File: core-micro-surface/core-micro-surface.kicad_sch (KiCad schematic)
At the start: 140 parts, among them J1 SWD, J2 AudioPlug2, J3 USB_B, J4 Screw_Terminal_01x04, SW1 SW_Push, SW10 SW_Push, SW11 SW_Push, SW12 SW_Push, SW13 SW_Push, SW14 SW_Push, SW15 SW_Push, SW16 SW_Push, SW17 SW_Push, SW18 SW_Push, SW19 SW_Push, SW2 SW_Push, SW20 SW_Push, SW21 SW_Push, SW22 SW_Push, SW23 SW_Push, SW24 SW_Push, SW25 SW_Push, SW26 SW_Push, SW27 SW_Push, SW28 SW_Push, SW29 SW_Push, SW3 SW_Push, SW30 SW_Push, SW31 SW_Push, SW32 SW_Push, SW33 SW_Push, SW34 SW_Push, SW35 SW_Push, SW36 SW_Push, SW37 SW_Push, SW38 SW_Push, SW39 SW_Push, SW4 SW_Push, SW40 SW_Push, SW41 SW_Push, SW42 SW_Push, SW43 SW_Push, SW44 SW_Push, SW45 SW_Push, SW46 RotaryEncoder_Switch, SW47 RotaryEncoder_Switch, SW48 RotaryEncoder_Switch, SW5 SW_Push, SW6 SW_Push, SW7 SW_Push, SW8 SW_Push, SW9 SW_Push, U1 RP2040, U2 W25Q128JVS, U3 XC6206PxxxMR-Regulator_Linear, U4 USBLC6-2SC6, U5 ADS1115IDGS, Y1 12MHz

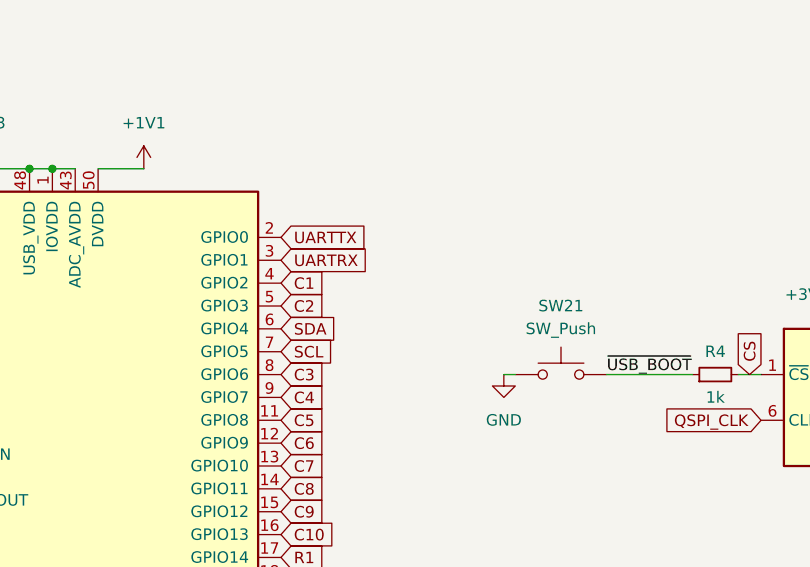
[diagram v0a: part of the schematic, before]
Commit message: Various things were completed
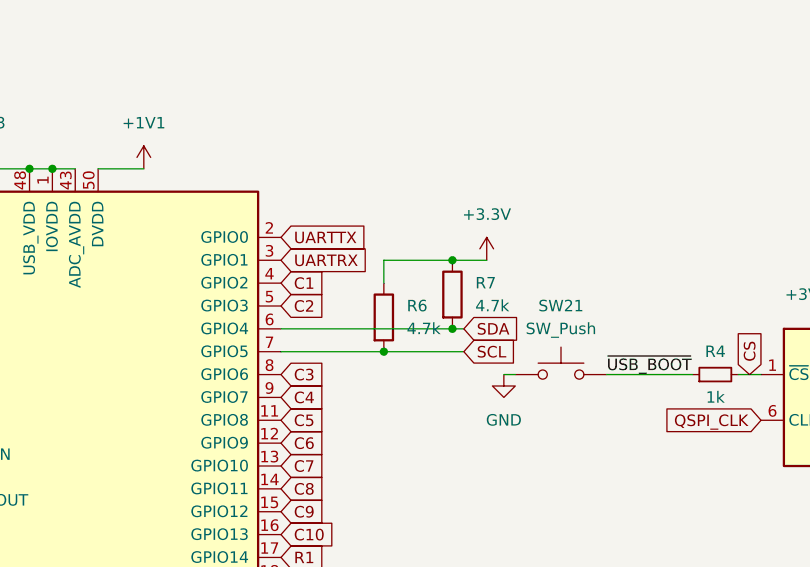
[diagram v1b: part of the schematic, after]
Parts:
- added R6, R7: 4.7k, Resistor_SMD:R_0402_1005Metric, symbol Device:R
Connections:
- net +3.3V: now also R6.1, R7.1
- net SCL: now also R6.2
- net SDA: now also R7.2
